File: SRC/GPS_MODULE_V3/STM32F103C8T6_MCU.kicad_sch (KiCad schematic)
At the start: 31 parts, among them J8 Conn_01x06, U2 STM32F103C8Tx, Y1 8MHz, Y2 32.678KHz

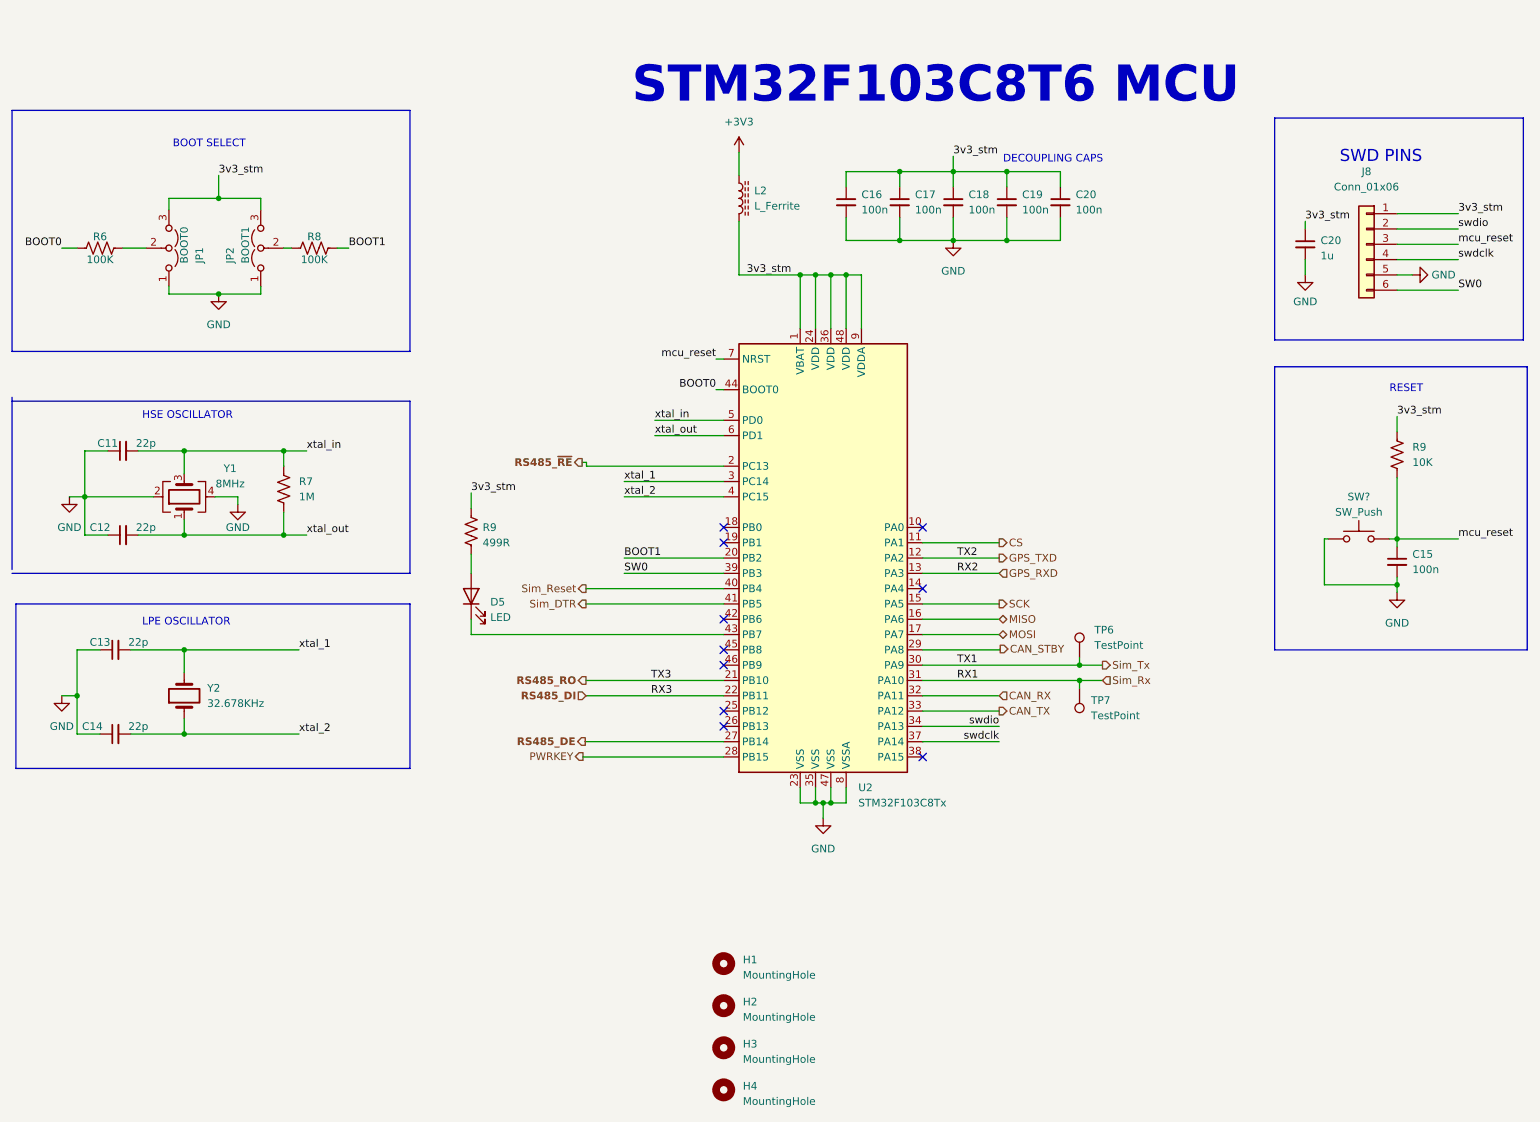
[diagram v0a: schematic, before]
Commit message: layut completed
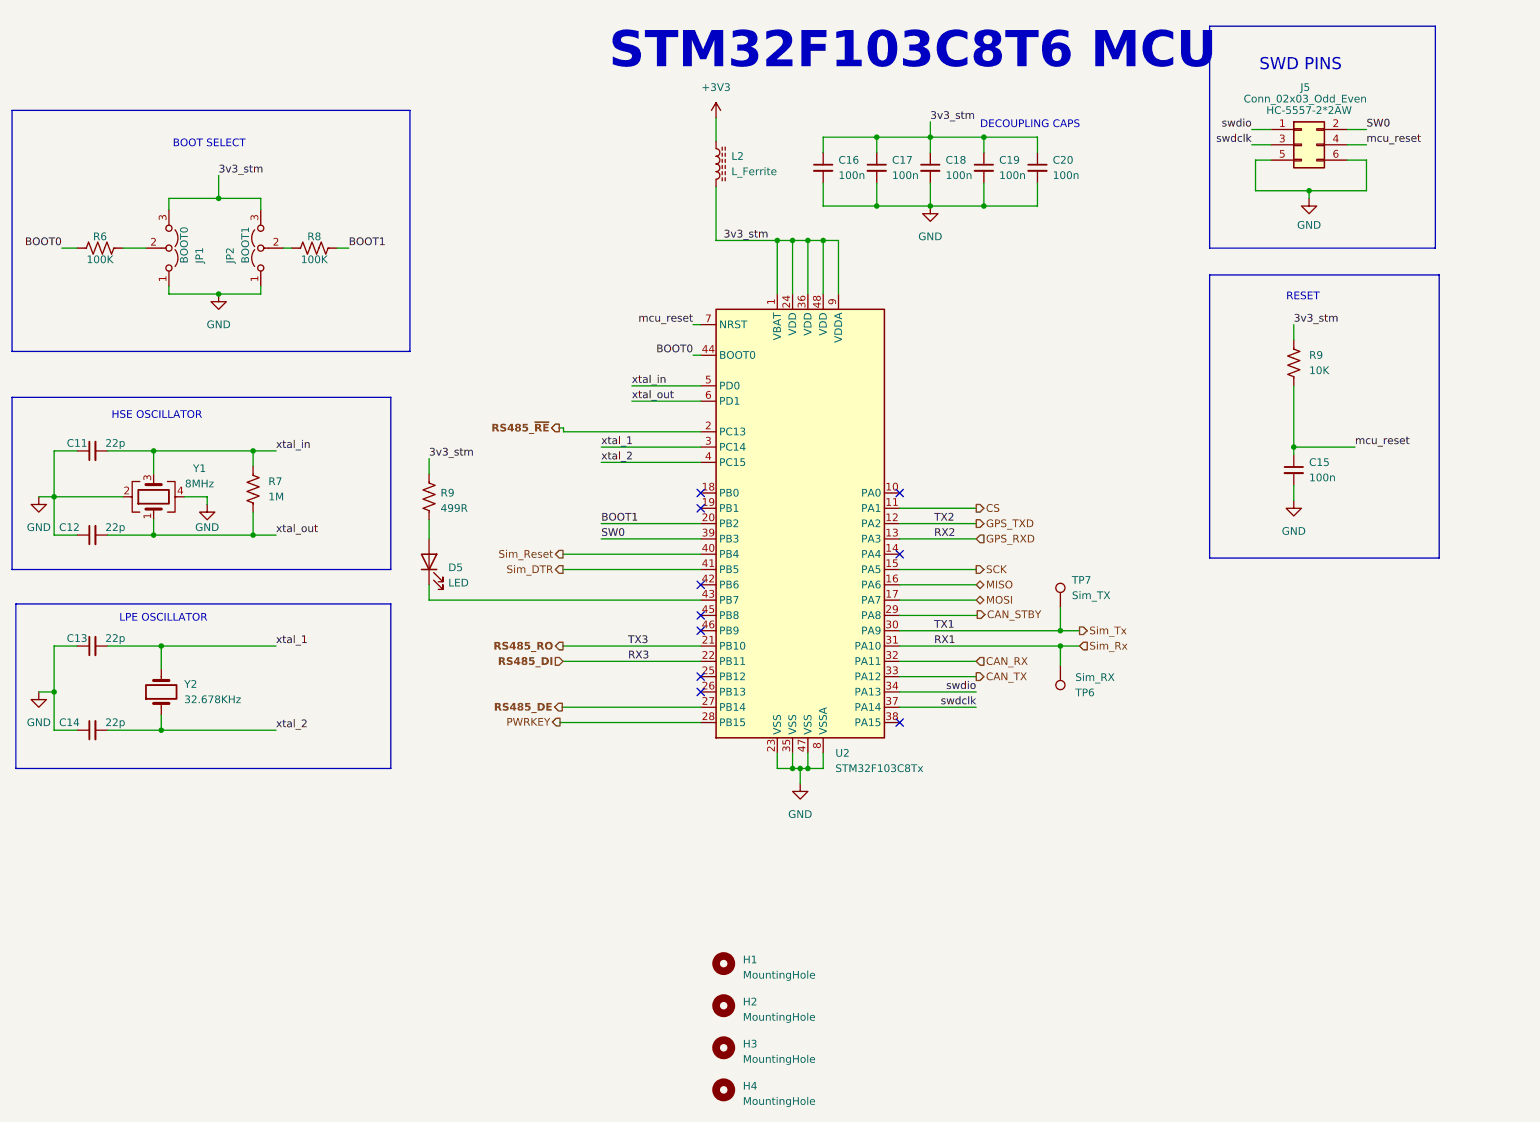
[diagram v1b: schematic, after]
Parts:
- removed C20: 1u, Capacitor_SMD:C_0402_1005Metric, symbol Device:C_Small
- removed J8: Conn_01x06, greencharge-footprints:J-LINK_6-PIN_NEEDLE_ADAPTER, symbol Connector_Generic:Conn_01x06
- removed SW?: SW_Push, greencharge-footprints:SKRPACE010, symbol Switch:SW_Push
- added J5: Conn_02x03_Odd_Even, Connector_Molex:Molex_Mini-Fit_Jr_5569-06A2_2x03_P4.20mm_Horizontal, symbol Connector_Generic:Conn_02x03_Odd_Even
- TP6: value TestPoint -> Sim_RX
- TP7: value TestPoint -> Sim_TX
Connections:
- net GND: now also J5.5 (Pin_5), J5.6 (Pin_6)
- net SW0: now also J5.2 (Pin_2)
- net Sim_Rx: now also TP6.1; no longer TP7.1
- net Sim_Tx: now also TP7.1; no longer TP6.1
- net mcu_reset: now also J5.4 (Pin_4)
- net swdclk: now also J5.3 (Pin_3)
- net swdio: now also J5.1 (Pin_1)
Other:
- moved on the sheet: C11, C12, C13, C14, C15, C16, C17, C18, C19, C20, D5, L2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
